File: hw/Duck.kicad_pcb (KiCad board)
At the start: 2 copper layers, 33.1 x 16.3 mm, 41 parts, among them J1 Conn_01x06, J2 Conn_01x06, J3 USB_C_Receptacle_USB2.0_14P, Q1 MMBT3904, Q2 MMBT3904, U1 ESP32-S3-PICO-1, U2 SPX3819M5-L-3-3, U3 INMP441, U4 MAX17048G+T10, U5 CH343P, U6 SPX3819M5-L-3-3

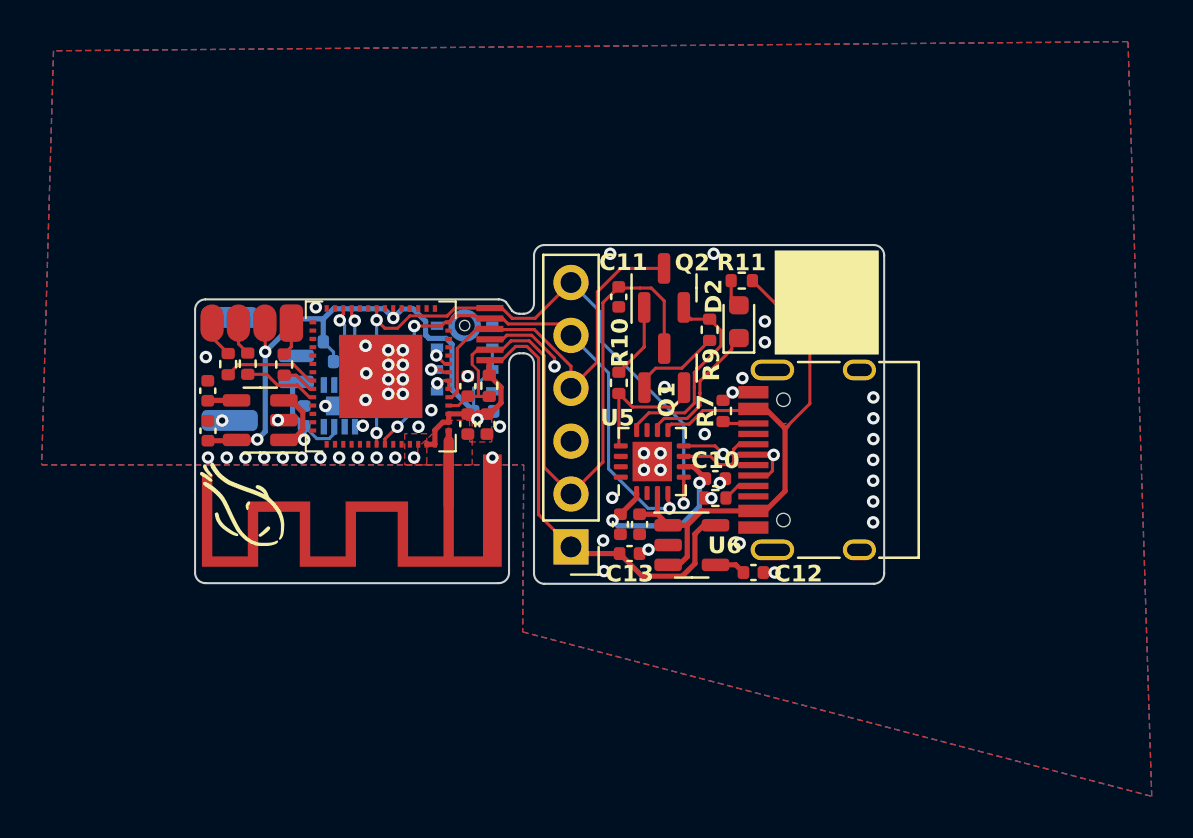
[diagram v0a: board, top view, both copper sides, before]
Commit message: hw: Hopefully all finished; polish in the details to-do
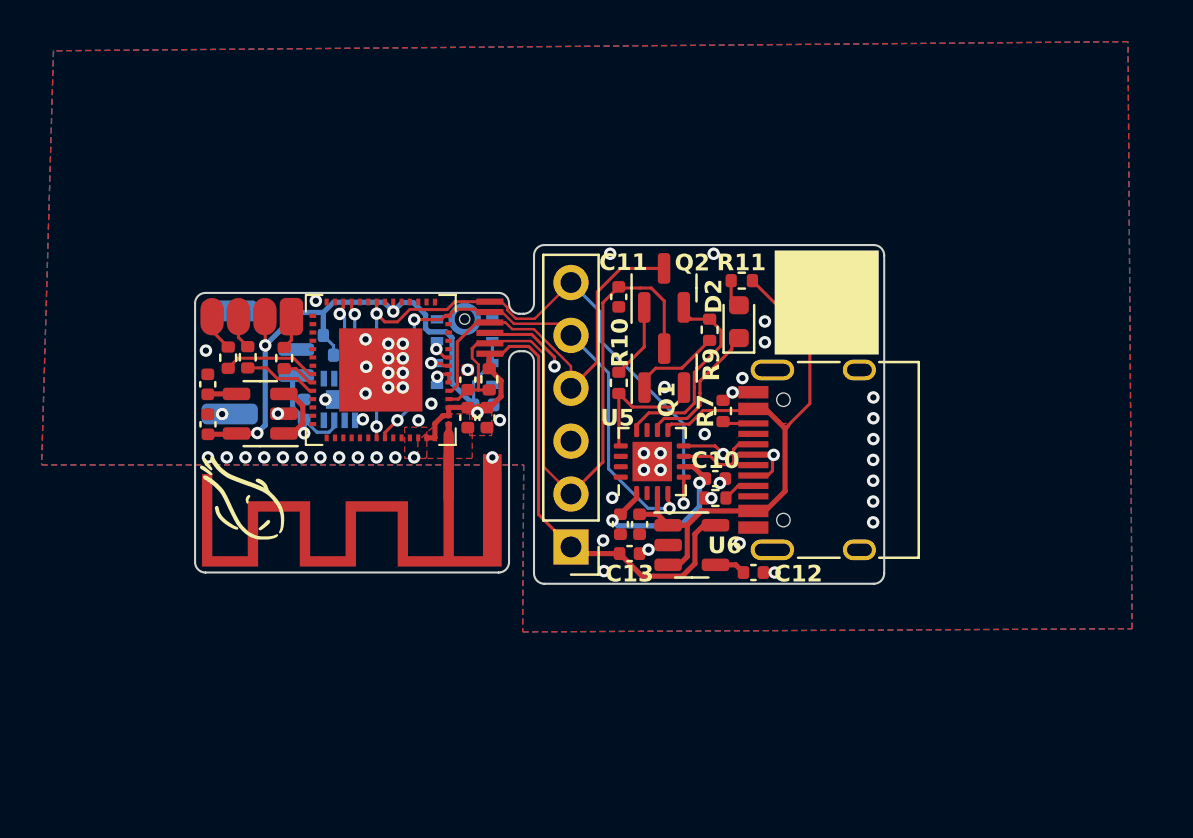
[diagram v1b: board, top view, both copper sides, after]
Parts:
- moved BT1 0.31 mm to (62.1, 44.8)
- moved C1 0.31 mm to (73.1, 47.5)
- moved C2 0.31 mm to (72.2, 47.5)
- moved C3 0.31 mm to (72.2, 45.6)
- moved C4 0.31 mm to (59.7, 45.9)
- moved C5 0.31 mm to (59.7, 47.8)
- moved C6 0.31 mm to (72.9, 46.9)
- moved C7 0.31 mm to (64.3, 47.1)
- moved D1 0.31 mm to (61.8, 42.6)
- moved G*** 0.31 mm to (61.3, 51.2)
- moved J1 0.31 mm to (73.2, 43.1)
- moved R3 0.31 mm to (66.2, 44.5)
- moved R4 0.31 mm to (63.3, 44.6)
- moved R5 0.31 mm to (61.6, 44.6)
- moved U1 0.31 mm to (68.0, 45.2)
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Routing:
- net /U0RXD: track 25.6 -> 26.4 mm
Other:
- outline, holes or cut-outs redrawn
